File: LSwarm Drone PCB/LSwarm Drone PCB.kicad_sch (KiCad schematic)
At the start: 128 parts, among them J1 Conn_01x04_Pin, J2 USB_C_Receptacle_USB2.0_16P, J3 JST / BT2.0 Connector, J4 Conn_01x02_Pin, J5 Conn_01x02_Pin, J6 Conn_01x02_Pin, J7 Conn_01x02_Pin, Q1 AO3400A, Q2 AO3400A, Q3 AO3400A, Q4 AO3400A, Q7 AO3407A, SW1 MSK12C02, U10 LSM6DSR, U11 BMP581, U12 AP2112K-3.3, U13 TPS61023DRLR, U14 SN74LVC1T45DBVR, Y1 12MHz, Y3 40MHz

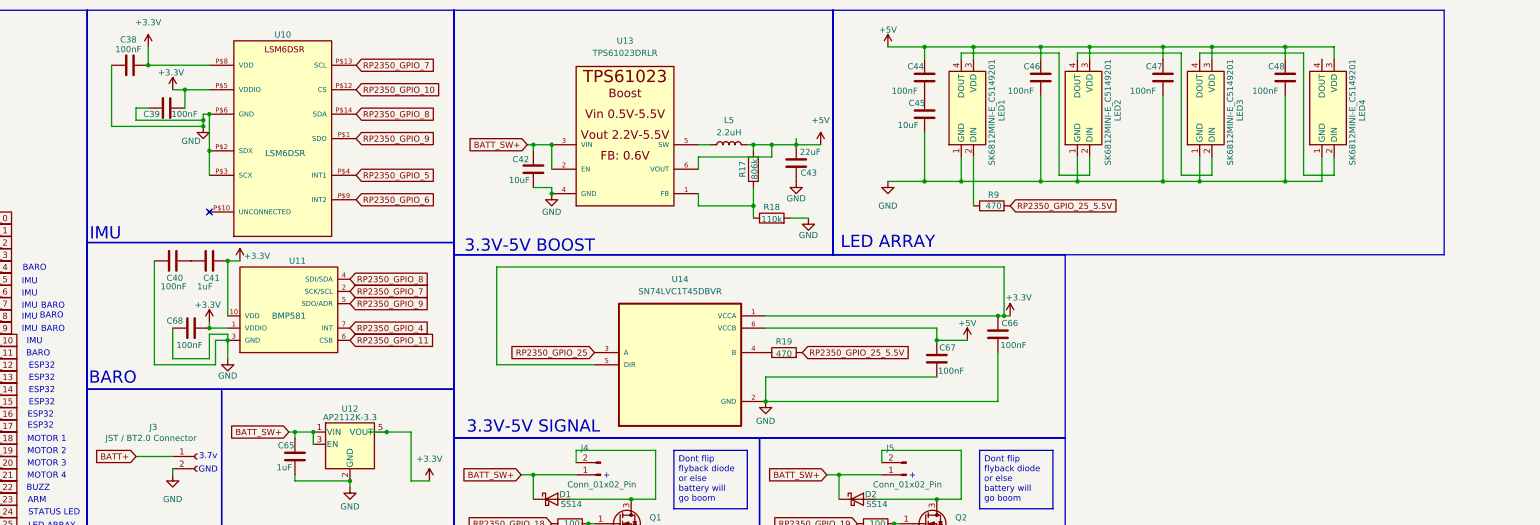
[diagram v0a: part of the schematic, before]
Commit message: sync
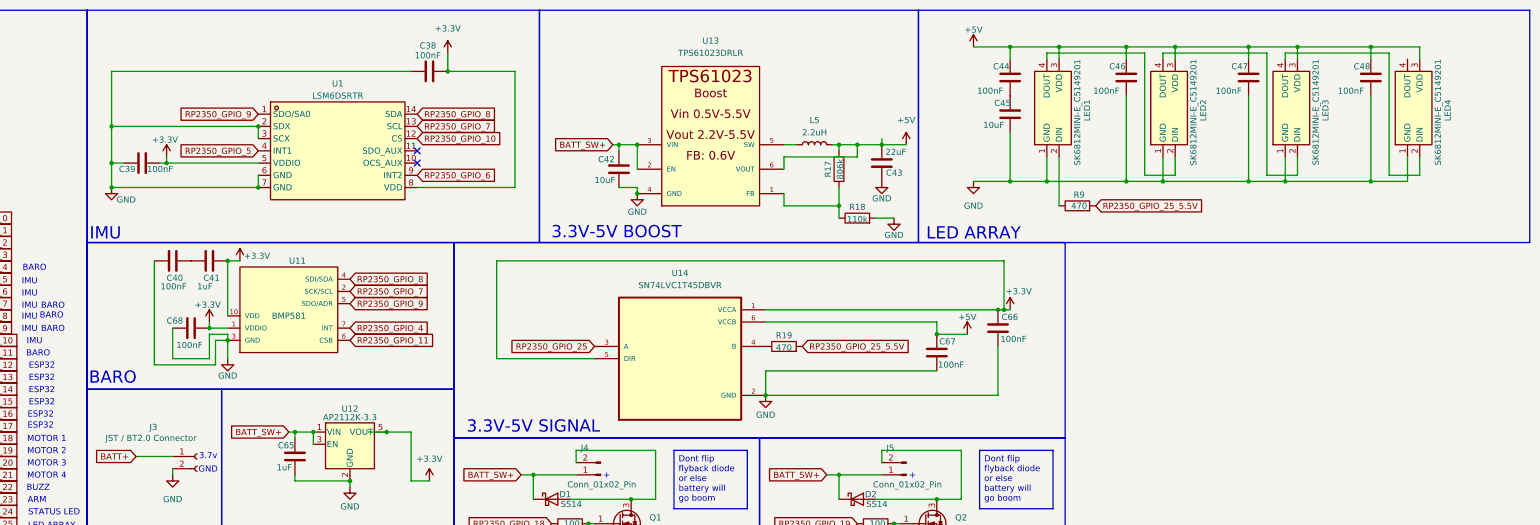
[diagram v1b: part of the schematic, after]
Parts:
- removed U10: LSM6DSR, LSM6DSR:LGA-14L, symbol LSM6DSR:LSM6DSR
- added U1: LSM6DSRTR, easyeda2kicad:LGA-14_L3.0-W2.5-P0.50-BR, symbol easyeda2kicad:LSM6DSRTR
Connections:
- net +3.3V: now also U1.5 (VDDIO), U1.8 (VDD)
- net GND: now also U1.2 (SDX), U1.3 (SCX), U1.6 (GND), U1.7 (GND)
- net RP2350_GPIO_10: now also U1.12 (CS)
- net RP2350_GPIO_5: now also U1.4 (INT1)
- net RP2350_GPIO_6: now also U1.9 (INT2)
- net RP2350_GPIO_7: now also U1.13 (SCL)
- net RP2350_GPIO_8: now also U1.14 (SDA)
- net RP2350_GPIO_9: now also U1.1 (SDO/SA0)
- no-connect marks 30 -> 31
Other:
- moved on the sheet: C38, C39, C42, C43, C44, C45, C46, C47, C48, C66, C67, L5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

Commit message: sync
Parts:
- removed ANT2: ANT3216LL00R2400A, ANT3216LL00R2400A:ANTC3216X135N, symbol ANT3216LL00R2400A:ANT3216LL00R2400A
- removed C25: 10nF, Capacitor_SMD:C_0603_1608Metric, symbol Device:C
- removed J2: USB_C_Receptacle_USB2.0_16P, Connector_USB:USB_C_Receptacle_HRO_TYPE-C-31-M-12, symbol Connector:USB_C_Receptacle_USB2.0_16P
- removed R1, R2: 5.1k, Resistor_SMD:R_0603_1608Metric, symbol Device:R
- removed R4, R5: 27, Resistor_SMD:R_0603_1608Metric, symbol Device:R
- removed S2, S3, S5, S6: SKRPACE010, SKRPACE010:SW_SKRPACE010, symbol SKRPACE010:SKRPACE010
- removed U11: BMP581, BMP581:BMP581, symbol BMP581:BMP581
- removed U13: TPS61023DRLR, TPS61023DRLR:SOT563-ORI, symbol TPS61023DRLR:TPS61023DRLR
- removed U14: SN74LVC1T45DBVR, SN74LVC1T45DBVR:SOT95P280X145-6N, symbol SN74LVC1T45DBVR:SN74LVC1T45DBVR
- added C26: 10nF, Capacitor_SMD:C_0603_1608Metric, symbol Device:C
- added JP1: U.FL-R-SMT-1, easyeda2kicad:RF-SMD_FRF05002-JSS103M, symbol easyeda2kicad:U.FL-R-SMT-1
- added R29, R30, R31: 10k, Resistor_SMD:R_0603_1608Metric, symbol Device:R
- added R32, R33: 5.1k, Resistor_SMD:R_0603_1608Metric, symbol Device:R
- added R34, R35: 27, Resistor_SMD:R_0603_1608Metric, symbol Device:R
- added SW2, SW3, SW4, SW5: SKRPACE010, easyeda2kicad:KEY-SMD_4P-L4.2-W3.2-P2.20-LS4.6, symbol easyeda2kicad:SKRPACE010
- added U3: TPS61023DRLR, easyeda2kicad:SOT-563_L1.6-W1.2-P0.50-LS1.6-BR, symbol easyeda2kicad:TPS61023DRLR
- added U4: SN74LVC1T45DBVR, easyeda2kicad:SOT-23-6_L2.9-W1.6-P0.95-LS2.8-BR, symbol easyeda2kicad:SN74LVC1T45DBVR
- added U5: BMP581, easyeda2kicad:LGA-10_L2.0-W2.0-P0.50-TL_BMP581, symbol easyeda2kicad:BMP581
- added USB1: USB-TYPE-C-018, easyeda2kicad:USB-C_SMD-TYPE-C-31-M-12, symbol easyeda2kicad:USB-TYPE-C-018
- renumbered FLASH to FLASH1, LED1 to STATUS1
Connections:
- net +3.3V: now also C40.2, R30.1, R31.1, U4.1 (VCCA), U4.5 (DIR), U5.1 (VDDIO), U5.10 (VDD); no longer C41.1
- net +5V: now also U3.6 (VOUT), U4.6 (VCCB)
- net BATT_SW+: now also U3.2 (EN), U3.3 (VIN)
- net GND: now also C41.1, R18.1, C26.1, JP1.2 (GND), JP1.3 (GND), R29.1, R32.2, R33.1, SW3.4, SW4.4, SW5.4, U3.4 (GND), U4.2 (GND), U5.3 (VSS), U5.8 (VSS), U5.9 (VSS), USB1.A1 (GND), USB1.A12 (GND), USB1.B1 (GND), USB1.B12 (GND); no longer C40.2, R18.2
- net RP2350_GPIO_10: now also R31.2
- net RP2350_GPIO_11: now also R30.2, U5.6 (CSB)
- net RP2350_GPIO_14: now also SW4.1
- net RP2350_GPIO_15: now also SW5.1
- net RP2350_GPIO_25: now also U4.3 (A)
- net RP2350_GPIO_4: now also U5.7 (INT)
- net RP2350_GPIO_5: now also R29.2
- net RP2350_GPIO_7: now also U5.2 (SCK)
- net RP2350_GPIO_8: now also U5.4 (SDI)
- net RP2350_GPIO_9: now also U5.5 (SDO)
- net RP2350_USB_DM: now also R34.2
- net RP2350_USB_DP: now also R35.1
- net at R17.1: now also R18.2, U3.1 (FB); no longer R18.1
- net at R3.2: now also SW3.1
- net at C9.1, RP2350.26 (RUN): now also SW2.1
- net at R8.2: now also SW2.3
- net at R19.1: now also U4.4 (B)
- net at L5.1: now also U3.5 (SW)
- net at C61.1, L8.2: now also JP1.1 (SIG)
- new net: R35.2, USB1.A6 (DP1), USB1.B6 (DP2)
- new net: R32.1, USB1.A5 (CC1)
- new net: R34.1, USB1.A7 (DN1), USB1.B7 (DN2)
- new net: C26.2, USB1.0 (SH), USB1.1 (SH), USB1.2 (SH), USB1.3 (SH)
- new net: USB1.A4 (VBUS), USB1.A9 (VBUS), USB1.B4 (VBUS), USB1.B9 (VBUS)
- new net: R33.2, USB1.B5 (CC2)
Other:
- moved on the sheet: C40, C41, C42, C43, C66, C67, C68, L5, R17, R18, R19

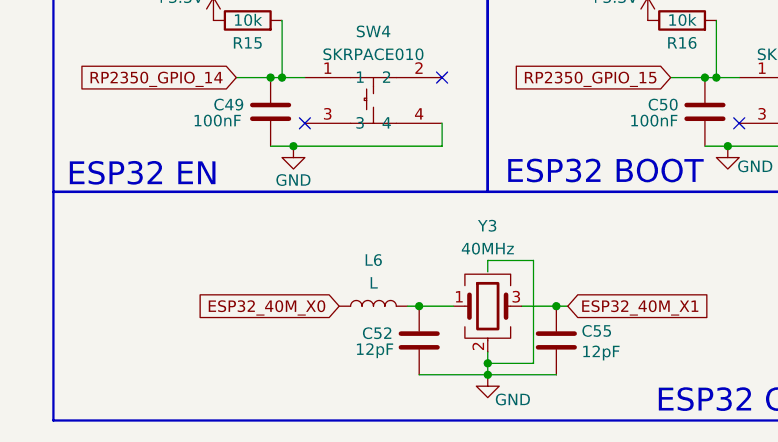
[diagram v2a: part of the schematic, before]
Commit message: sync
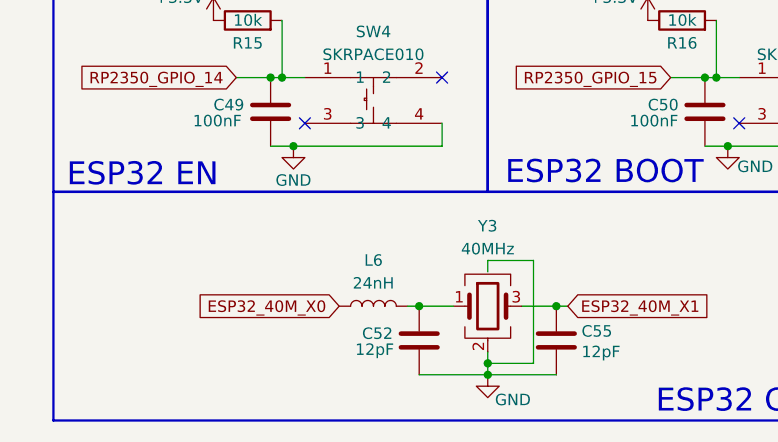
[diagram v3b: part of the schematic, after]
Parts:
- L6: value L -> 24nH
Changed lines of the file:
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@@
 			)
 		)
-		(property "Value" "L"
+		(property "Value" "24nH"
 			(at 48.26 261.62 90)
 			(show_name no)

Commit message: sync
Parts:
- removed C52, C55: 12pF, Capacitor_SMD:C_0603_1608Metric, symbol Device:C
- removed C72: 220uF, Capacitor_Tantalum_SMD:CP_EIA-3528-21_Kemet-B, symbol Device:C
- removed L6: 24nH, Inductor_SMD:L_0805_2012Metric, symbol Device:L
- removed R18: 110k, Resistor_SMD:R_0603_1608Metric, symbol Device:R
- removed Y1: 12MHz, Crystal:Crystal_SMD_3225-4Pin_3.2x2.5mm, symbol Device:Crystal_GND24
- removed Y3: 40MHz, Crystal:Crystal_SMD_3225-4Pin_3.2x2.5mm, symbol Device:Crystal_GND24
- added C1: CL21A226MAQNNNE, easyeda2kicad:C0805, symbol easyeda2kicad:CL21A226MAQNNNE
- added R36: 820k, Resistor_SMD:R_0603_1608Metric, symbol Device:R
- added R37: 100k, Resistor_SMD:R_0603_1608Metric, symbol Device:R
- added X1: X322512MSB4SI, easyeda2kicad:CRYSTAL-SMD_4P-L3.2-W2.5-BL, symbol easyeda2kicad:X322512MSB4SI
- R17: value 806k -> 10k
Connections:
- net +5V: now also R36.1; no longer R17.2
- net BATT_SW+: now also C1.1
- net GND: now also C7.1, C8.1, C1.2, R37.2, X1.2 (GND), X1.4 (GND); no longer C7.2, C8.2
- net RP2350_XIN: now also C8.2, X1.1 (OSC1); no longer C8.1
- net at R17.1: now also SW1.2; no longer U3.1 (FB)
- net at R7.1: now also C7.2, X1.3 (OSC2); no longer C7.1
- net at Q7.1 (G), R28.1: now also R17.2; no longer SW1.2
- new net: R36.2, R37.1, U3.1 (FB)
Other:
- note removed: "ESP32 CRYSTAL"
- moved on the sheet: C7, C71Ceramic1, C8, Q7, R28, R7
